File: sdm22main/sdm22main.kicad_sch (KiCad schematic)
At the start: 2 parts, among them U1 Teensy4.1

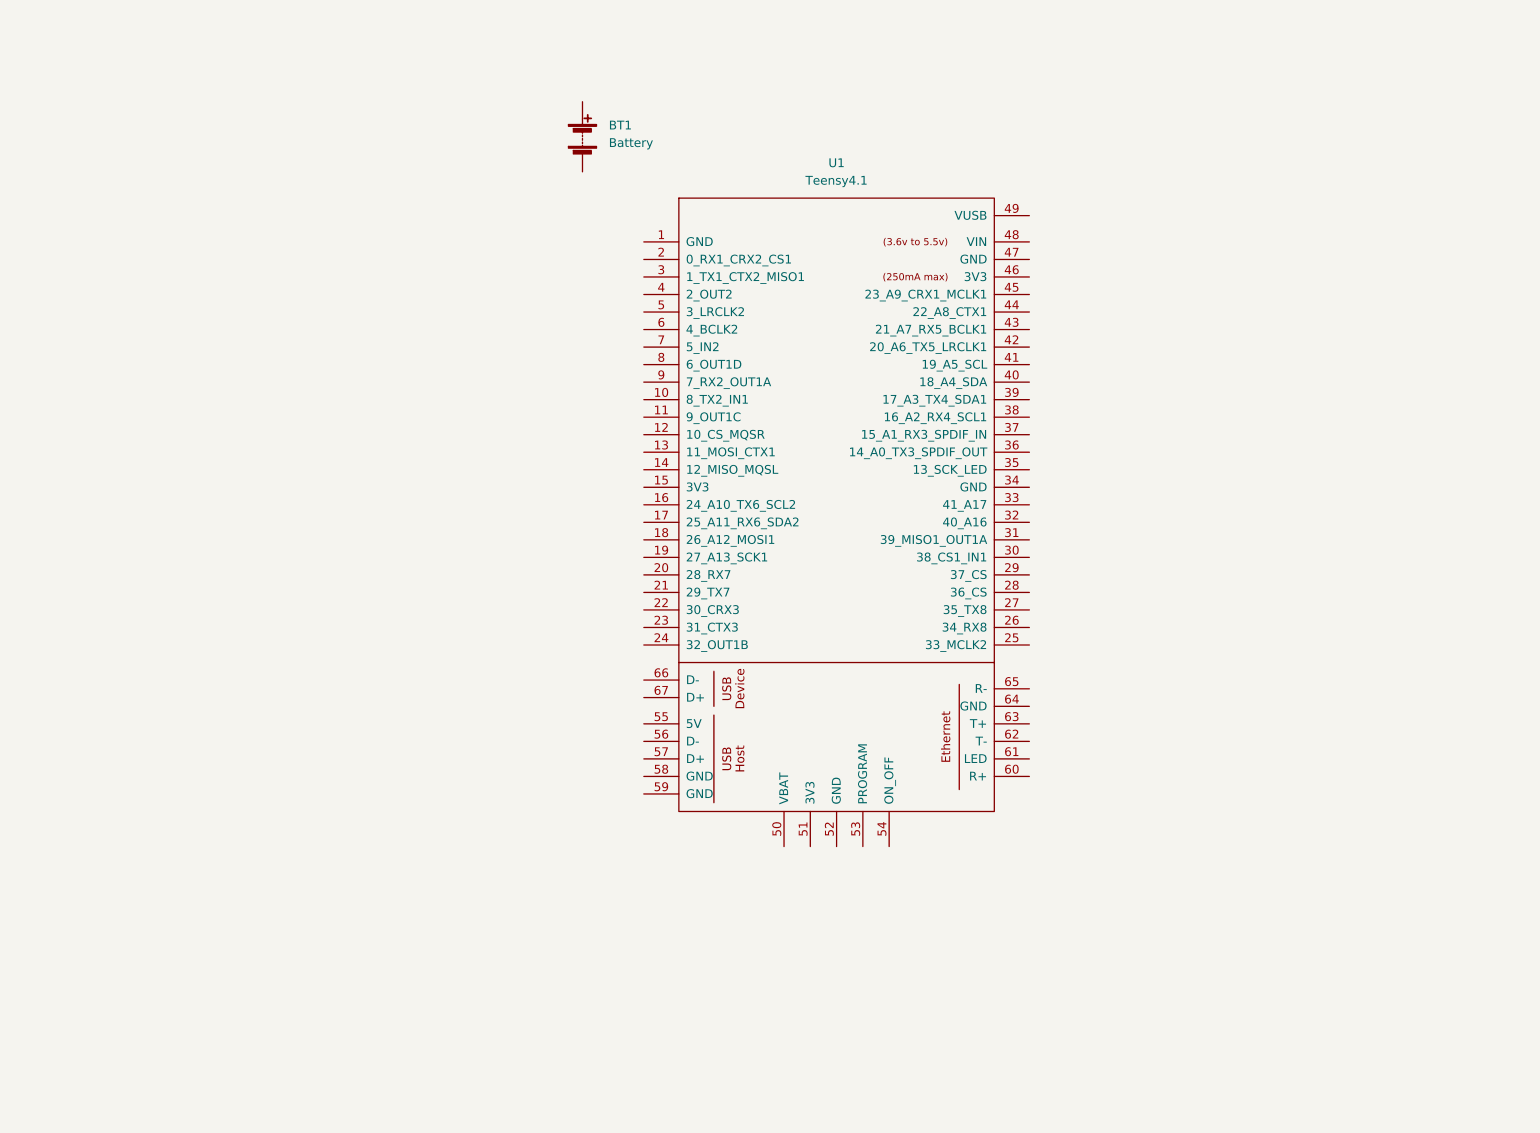
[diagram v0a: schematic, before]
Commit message: finished first draft of main board
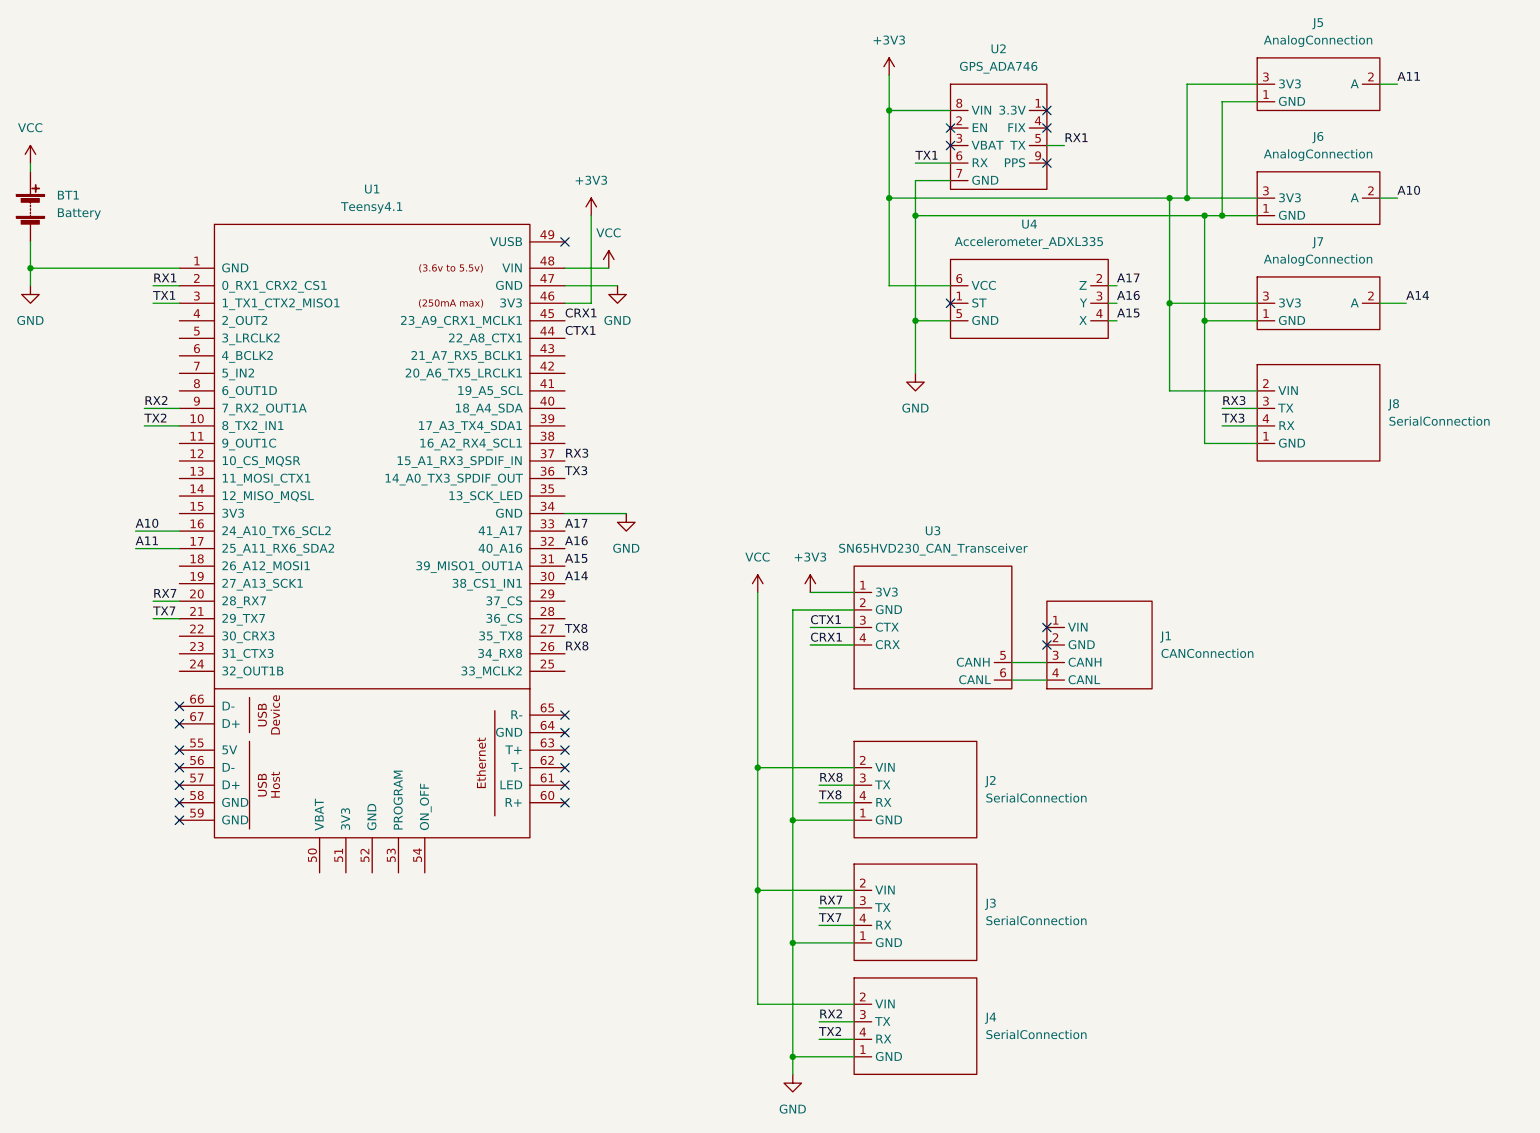
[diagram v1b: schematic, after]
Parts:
- added J1: CANConnection, symbol SDM:CANConnection
- added J2, J3, J4, J8: SerialConnection, SDM:4Wire_SerialConnector, symbol SDM:SerialConnection
- added J5, J6, J7: AnalogConnection, SDM:3Wire_AnalogConnector, symbol SDM:AnalogConnection
- added U2: GPS_ADA746, symbol SDM:GPS_ADA746
- added U3: SN65HVD230_CAN_Transceiver, symbol SDM:SN65HVD230_CAN_Transceiver
- added U4: Accelerometer_ADXL335, symbol SDM:Accelerometer_ADXL335
- BT1: footprint (none) -> Connector_PinSocket_2.54mm:PinSocket_1x02_P2.54mm_Vertical
- U1: footprint (none) -> Teensy:Teensy41
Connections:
- net VCC: now reaches BT1.1 (+)
- net VCC: now also U1.48 (VIN), J2.2 (VIN), J3.2 (VIN), J4.2 (VIN)
- net GND: now reaches BT1.2 (-)
- net GND: now also U1.1 (GND), U1.34 (GND), U1.47 (GND), J2.1 (GND), J3.1 (GND), J4.1 (GND), J5.1 (GND), J6.1 (GND), J7.1 (GND), J8.1 (GND), U2.7 (GND), U3.2 (GND), U4.5 (GND)
- net TX2: now reaches U1.10 (8_TX2_IN1)
- net TX2: now also J4.4 (RX)
- net A10: now reaches U1.16 (24_A10_TX6_SCL2)
- net A10: now also J6.2 (A)
- net A11: now reaches U1.17 (25_A11_RX6_SDA2)
- net A11: now also J5.2 (A)
- net RX1: now reaches U1.2 (0_RX1_CRX2_CS1)
- net RX1: now also U2.5 (TX)
- net RX7: now reaches U1.20 (28_RX7)
- net RX7: now also J3.3 (TX)
- net TX7: now reaches U1.21 (29_TX7)
- net TX7: now also J3.4 (RX)
- net RX8: now reaches U1.26 (34_RX8)
- net RX8: now also J2.3 (TX)
- net TX8: now reaches U1.27 (35_TX8)
- net TX8: now also J2.4 (RX)
- net TX1: now reaches U1.3 (1_TX1_CTX2_MISO1)
- net TX1: now also U2.6 (RX)
- net A14: now reaches U1.30 (38_CS1_IN1)
- net A14: now also J7.2 (A)
- net A15: now reaches U1.31 (39_MISO1_OUT1A)
- net A15: now also U4.4 (X)
- net A16: now reaches U1.32 (40_A16)
- net A16: now also U4.3 (Y)
- net A17: now reaches U1.33 (41_A17)
- net A17: now also U4.2 (Z)
- net TX3: now reaches U1.36 (14_A0_TX3_SPDIF_OUT)
- net TX3: now also J8.4 (RX)
- net RX3: now reaches U1.37 (15_A1_RX3_SPDIF_IN)
- net RX3: now also J8.3 (TX)
- net CTX1: now reaches U1.44 (22_A8_CTX1)
- net CTX1: now also U3.3 (CTX)
- net CRX1: now reaches U1.45 (23_A9_CRX1_MCLK1)
- net CRX1: now also U3.4 (CRX)
- net +3V3: now reaches U1.46 (3V3)
- net +3V3: now also J5.3 (3V3), J6.3 (3V3), J7.3 (3V3), J8.2 (VIN), U2.8 (VIN), U3.1 (3V3), U4.6 (VCC)
- net RX2: now reaches U1.9 (7_RX2_OUT1A)
- net RX2: now also J4.3 (TX)
- new net: J1.3 (CANH), U3.5 (CANH)
- new net: J1.4 (CANL), U3.6 (CANL)
- no-connect marks 0 -> 22
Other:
- moved on the sheet: BT1, U1
